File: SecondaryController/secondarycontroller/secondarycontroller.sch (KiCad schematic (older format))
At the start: 9 parts, among them J1 Receiver, J2 Conn_01x07_Female, J3 VIN, J4 APA102C, J5 I2C BUS, SW1 Calibrate, SW2 Reset

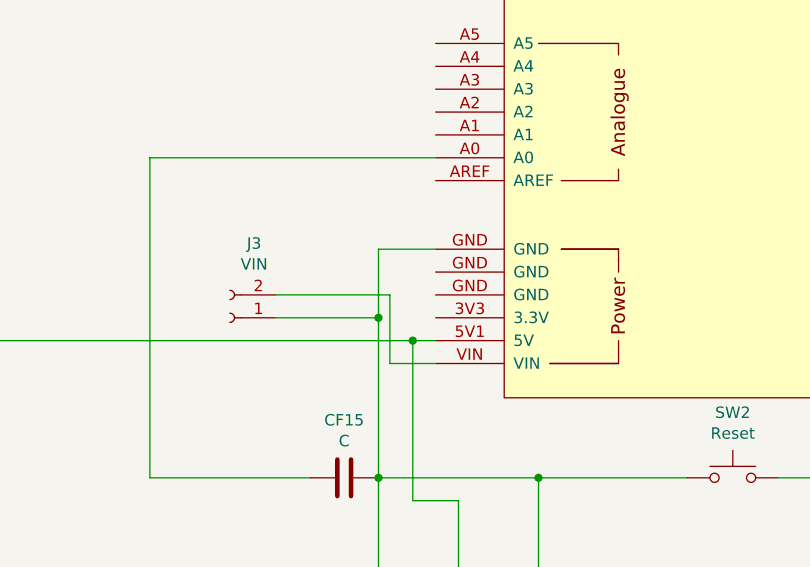
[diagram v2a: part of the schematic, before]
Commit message: secondary as done
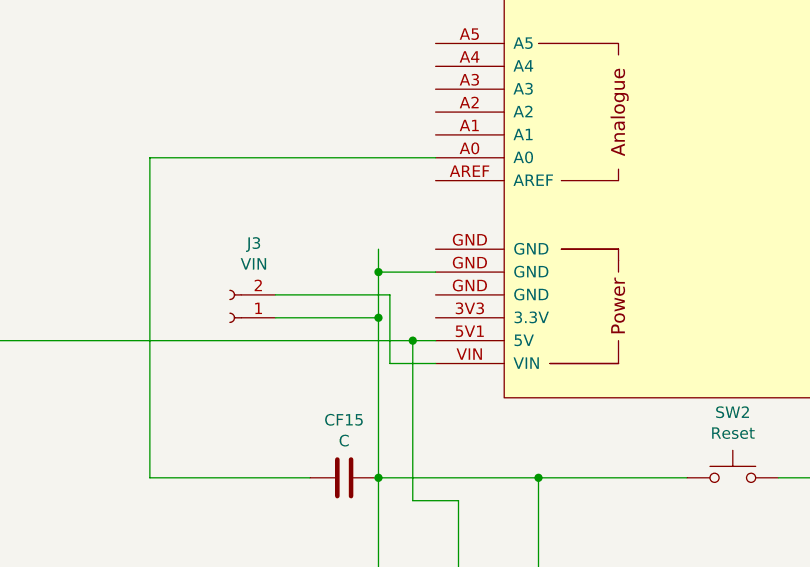
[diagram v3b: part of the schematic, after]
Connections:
- net at XA1.GND: now also CF15.1, J1.1 (Pin_1), J2.2 (Pin_2), J2.6 (Pin_6), J3.1 (Pin_1), J4.1 (Pin_1), SW1.2, SW2.1
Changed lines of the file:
@@
 	2100 3600 2550 3600
 Wire Wire Line
-	2550 3600 2550 3300
-Wire Wire Line
-	2550 3300 2800 3300
+	2550 3600 2550 3400
 $Comp
 L secondarycontroller-rescue:C-Device CF15
@@
 Wire Wire Line
 	5700 1700 6050 1700
+Wire Wire Line
+	2800 3400 2550 3400
+Connection ~ 2550 3400
+Wire Wire Line
+	2550 3400 2550 3300
 $EndSCHEMATC

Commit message: new secondary controller pcb design
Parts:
- added D1: DIODE, Diode_THT:D_5W_P12.70mm_Horizontal, symbol pspice:DIODE
- added Potentiometer1: Conn_01x03_Male, Connector_JST:JST_EH_B03B-EH-A_1x03_P2.50mm_Vertical, symbol Connector:Conn_01x03_Male
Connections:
- wire segments 74 -> 81
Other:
- moved on the sheet: J3
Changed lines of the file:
@@
 $EndComp
-$Comp
-L secondarycontroller-rescue:Conn_01x02_Female-Connector J3
-U 1 1 5BBE53F0
-P 1900 3600
-F 0 "J3" H 1794 3275 50  0000 C CNN
-F 1 "VIN" H 1794 3366 50  0000 C CNN
-F 2 "Connector_PinHeader_2.54mm:PinHeader_1x02_P2.54mm_Vertical" H 1900 3600 50  0001 C CNN
-F 3 "~" H 1900 3600 50  0001 C CNN
-	1    1900 3600
-	-1   0    0    1
-$EndComp
-Wire Wire Line
-	2100 3500 2600 3500
-Wire Wire Line
-	2600 3500 2600 3800
-Wire Wire Line
-	2600 3800 2800 3800
-Wire Wire Line
-	2100 3600 2550 3600
-Wire Wire Line
-	2550 3600 2550 3400
 $Comp
 L secondarycontroller-rescue:C-Device CF15
@@
 Wire Wire Line
 	3900 4300 3250 4300
-Connection ~ 2550 3600
-Wire Wire Line
-	2550 4300 2550 3600
 Wire Wire Line
 	2800 3700 2700 3700
@@
 	2900 4400 2900 5400
 Wire Wire Line
-	700  3700 2700 3700
+	700  3700 2200 3700
 Connection ~ 2700 3700
 Wire Wire Line
@@
 Connection ~ 2550 4300
 Wire Wire Line
-	2800 2900 1550 2900
+	2800 2900 2300 2900
 Wire Wire Line
 	1550 2900 1550 4300
@@
 	2800 3400 2550 3400
 Connection ~ 2550 3400
-Wire Wire Line
-	2550 3400 2550 3300
+$Comp
+L Connector:Conn_01x03_Male Potentiometer1
+U 1 1 5BDD001F
+P 2000 2550
+F 0 "Potentiometer1" H 2106 2828 50  0000 C CNN
+F 1 "Conn_01x03_Male" H 2106 2737 50  0000 C CNN
+F 2 "Connector_JST:JST_EH_B03B-EH-A_1x03_P2.50mm_Vertical" H 2000 2550 50  0001 C CNN
+F 3 "~" H 2000 2550 50  0001 C CNN
+	1    2000 2550
+	1    0    0    -1
+$EndComp
+Wire Wire Line
+	2200 2450 2550 2450
+Connection ~ 2200 3700
+Wire Wire Line
+	2200 3700 2700 3700
+Wire Wire Line
+	2300 2900 2300 2550
+Wire Wire Line
+	2300 2550 2200 2550
+Connection ~ 2300 2900
+Wire Wire Line
+	2300 2900 1550 2900
+$Comp
+L secondarycontroller-rescue:Conn_01x02_Female-Connector J3
+U 1 1 5BBE53F0
+P 1150 3200
+F 0 "J3" H 1044 2875 50  0000 C CNN
+F 1 "VIN" H 1044 2966 50  0000 C CNN
+F 2 "Connector_PinHeader_2.54mm:PinHeader_1x02_P2.54mm_Vertical" H 1150 3200 50  0001 C CNN
+F 3 "~" H 1150 3200 50  0001 C CNN
+	1    1150 3200
+	-1   0    0    1
+$EndComp
+$Comp
+L pspice:DIODE D1
+U 1 1 5BDD7261
+P 1900 3200
+F 0 "D1" H 1900 3465 50  0000 C CNN
+F 1 "DIODE" H 1900 3374 50  0000 C CNN
+F 2 "Diode_THT:D_5W_P12.70mm_Horizontal" H 1900 3200 50  0001 C CNN
+F 3 "" H 1900 3200 50  0001 C CNN
+	1    1900 3200
+	1    0    0    -1
+$EndComp
+Wire Wire Line
+	1350 3200 1700 3200
+Wire Wire Line
+	2100 3200 2550 3200
+Wire Wire Line
+	2550 2450 2550 3200
+Connection ~ 2550 3200
+Wire Wire Line
+	2550 3200 2550 3400
+Wire Wire Line
+	2550 3400 2550 4300
+Wire Wire Line
+	2200 2650 2200 3700
+Wire Wire Line
+	1350 3100 1650 3100
+Wire Wire Line
+	1650 3100 1650 3800
+Wire Wire Line
+	1650 3800 2800 3800
 $EndSCHEMATC
